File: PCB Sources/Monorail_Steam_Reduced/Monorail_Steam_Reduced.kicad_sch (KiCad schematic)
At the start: 130 parts, among them J1 Conn_01x02_Male, J2 Conn_01x02_Male, J3 Conn_01x02_Male, J6 USB_C_Receptacle_USB2.0, J8 Conn_01x04_Male, J9 Conn_01x03_Male, SW3 RotaryEncoder_Switch, U1 SRV05-4, U2 XC6206PxxxMR, U3 RP2040TR7, U4 W25Q128JVS, Y1 Crystal_GND24_Small

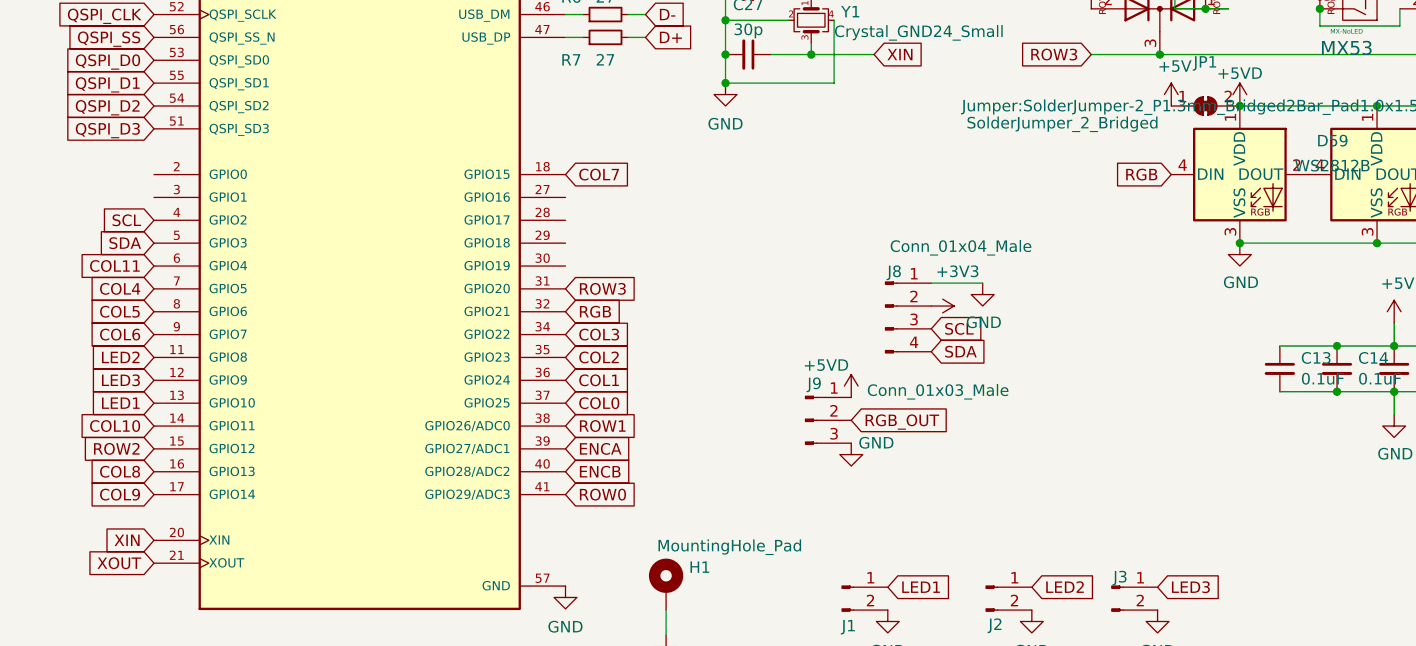
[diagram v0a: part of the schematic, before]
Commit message: finalized silkscreen and fixed positions
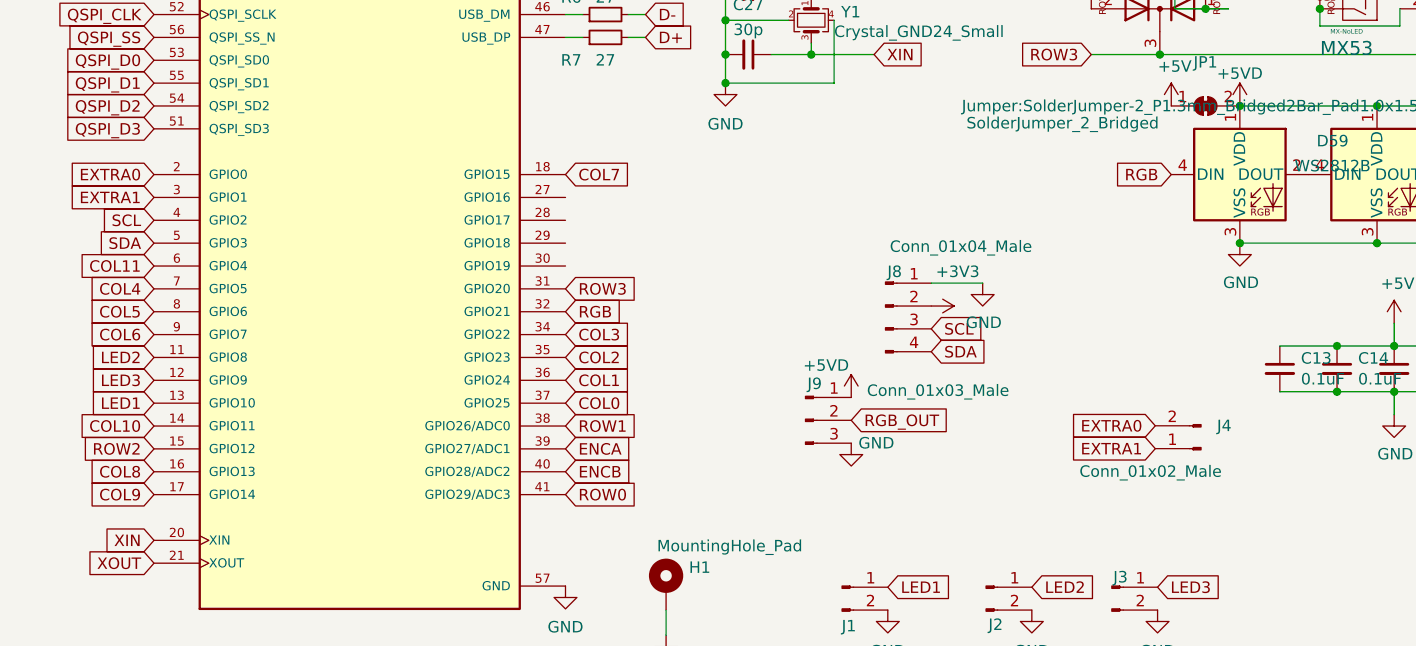
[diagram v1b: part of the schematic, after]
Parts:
- added J4: Conn_01x02_Male, Connector_PinSocket_2.54mm:PinSocket_1x02_P2.54mm_Vertical, symbol Connector:Conn_01x02_Male
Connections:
- net EXTRA0: now reaches U3.2 (GPIO0)
- net EXTRA0: now also J4.2 (Pin_2)
- net EXTRA1: now reaches U3.3 (GPIO1)
- net EXTRA1: now also J4.1 (Pin_1)
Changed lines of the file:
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@@
     (stroke (width 0) (type default))
   )
+  (global_label "EXTRA1" (shape input) (at 141.732 168.2496 180) (fields_autoplaced)
+    (effects (font (size 1.27 1.27)) (justify right))
+    (property "Intersheetrefs" "${INTERSHEET_REFS}" (at 132.5068 168.2496 0)
+      (effects (font (size 1.27 1.27)) (justify right) hide)
+    )
+  )
   (global_label "COL4" (shape input) (at 30.48 150.495 180) (fields_autoplaced)
     (effects (font (size 1.27 1.27)) (justify right))
@@
     )
   )
+  (global_label "EXTRA0" (shape input) (at 141.732 165.7096 180) (fields_autoplaced)
+    (effects (font (size 1.27 1.27)) (justify right))
+    (property "Intersheetrefs" "${INTERSHEET_REFS}" (at 132.5068 165.7096 0)
+      (effects (font (size 1.27 1.27)) (justify right) hide)
+    )
+  )
   (global_label "QSPI_D1" (shape input) (at 30.48 127.635 180) (fields_autoplaced)
     (effects (font (size 1.27 1.27)) (justify right))
@@
     )
   )
+  (global_label "EXTRA1" (shape input) (at 30.48 140.335 180) (fields_autoplaced)
+    (effects (font (size 1.27 1.27)) (justify right))
+    (property "Intersheetrefs" "${INTERSHEET_REFS}" (at 21.2548 140.335 0)
+      (effects (font (size 1.27 1.27)) (justify right) hide)
+    )
+  )
   (global_label "COL1" (shape input) (at 76.2 160.655 0) (fields_autoplaced)
     (effects (font (size 1.27 1.27)) (justify left))
@@
     (property "Intersheetrefs" "${INTERSHEET_REFS}" (at 83.3691 137.795 0)
       (effects (font (size 1.27 1.27)) (justify left) hide)
+    )
+  )
+  (global_label "EXTRA0" (shape input) (at 30.48 137.795 180) (fields_autoplaced)
+    (effects (font (size 1.27 1.27)) (justify right))
+    (property "Intersheetrefs" "${INTERSHEET_REFS}" (at 21.2548 137.795 0)
+      (effects (font (size 1.27 1.27)) (justify right) hide)
     )
   )
@@
         )
       )
+    )
+  )
+  (symbol (lib_id "Connector:Conn_01x02_Male") (at 146.812 168.2496 180) (unit 1)
+    (in_bom yes) (on_board yes) (dnp no)
+    (property "Reference" "J4" (at 148.59 165.7096 0)
+      (effects (font (size 1.27 1.27)) (justify right))
+    )
+    (property "Value" "Conn_01x02_Male" (at 133.2992 170.7896 0)
+      (effects (font (size 1.27 1.27)) (justify right))
+    )
+    (property "Footprint" "Connector_PinSocket_2.54mm:PinSocket_1x02_P2.54mm_Vertical" (at 146.812 168.2496 0)
+      (effects (font (size 1.27 1.27)) hide)
+    )
+    (property "Datasheet" "~" (at 146.812 168.2496 0)
+      (effects (font (size 1.27 1.27)) hide)
+    )
+    (pin "1")
+    (pin "2")
+    (instances
+      (project "Monorail_Steam_Reduced"
+        (path "/a3e4f0ae-9f86-49e9-b386-ed8b42e012fb"
+          (reference "J4") (unit 1)
+        )
+      )
